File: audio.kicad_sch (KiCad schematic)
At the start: 33 parts, among them IC1 ES9218PQ, J5 SJ2-35954B-SMT-TR, Y2 ECS-2520SMV-500-GP-TR

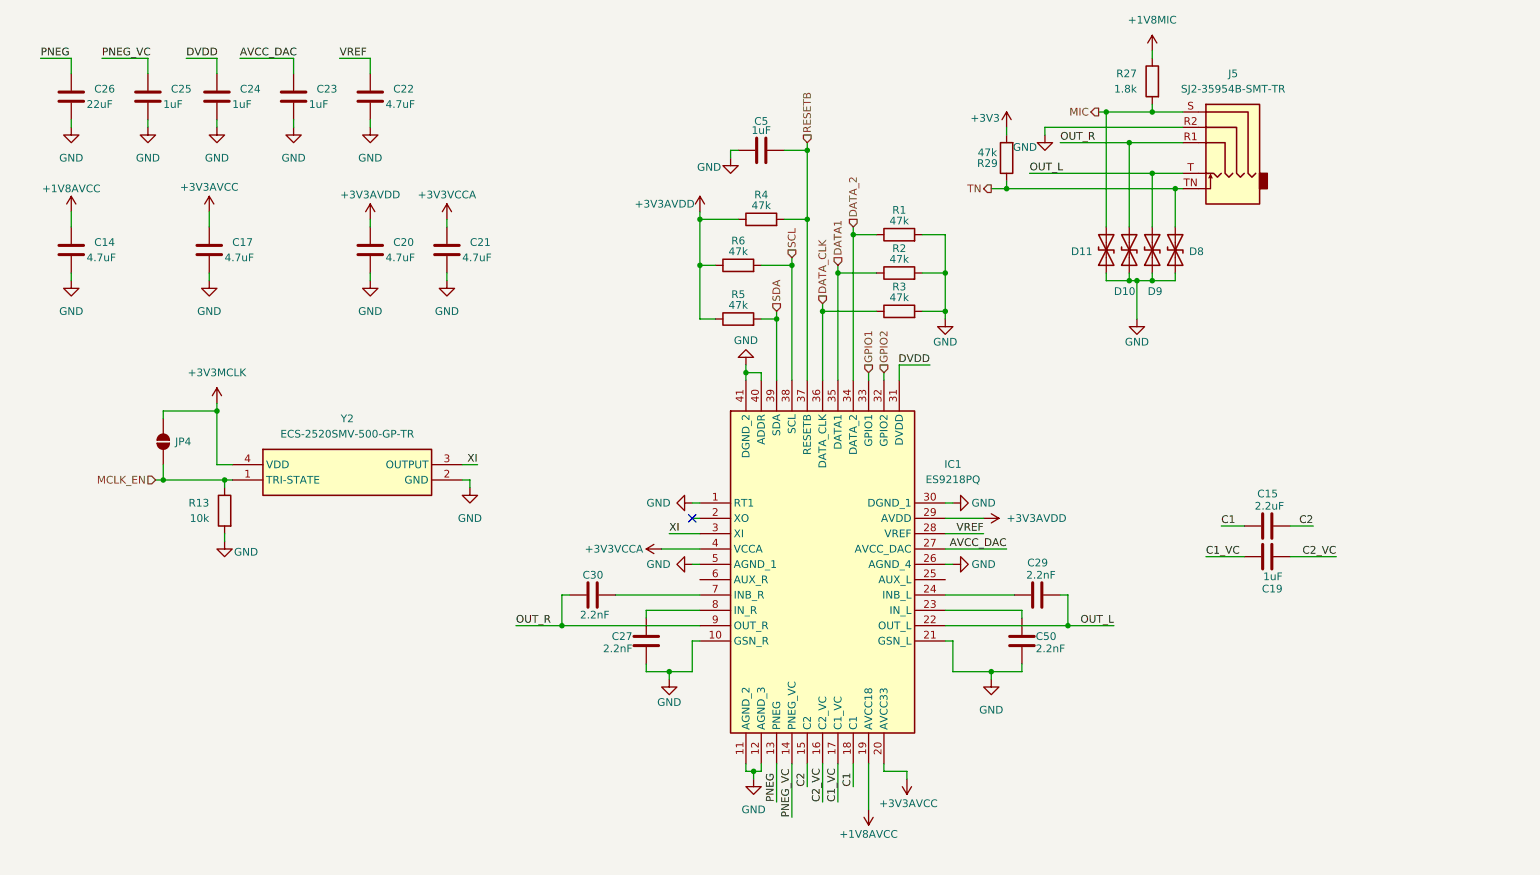
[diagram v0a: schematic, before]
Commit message: segmented schematci
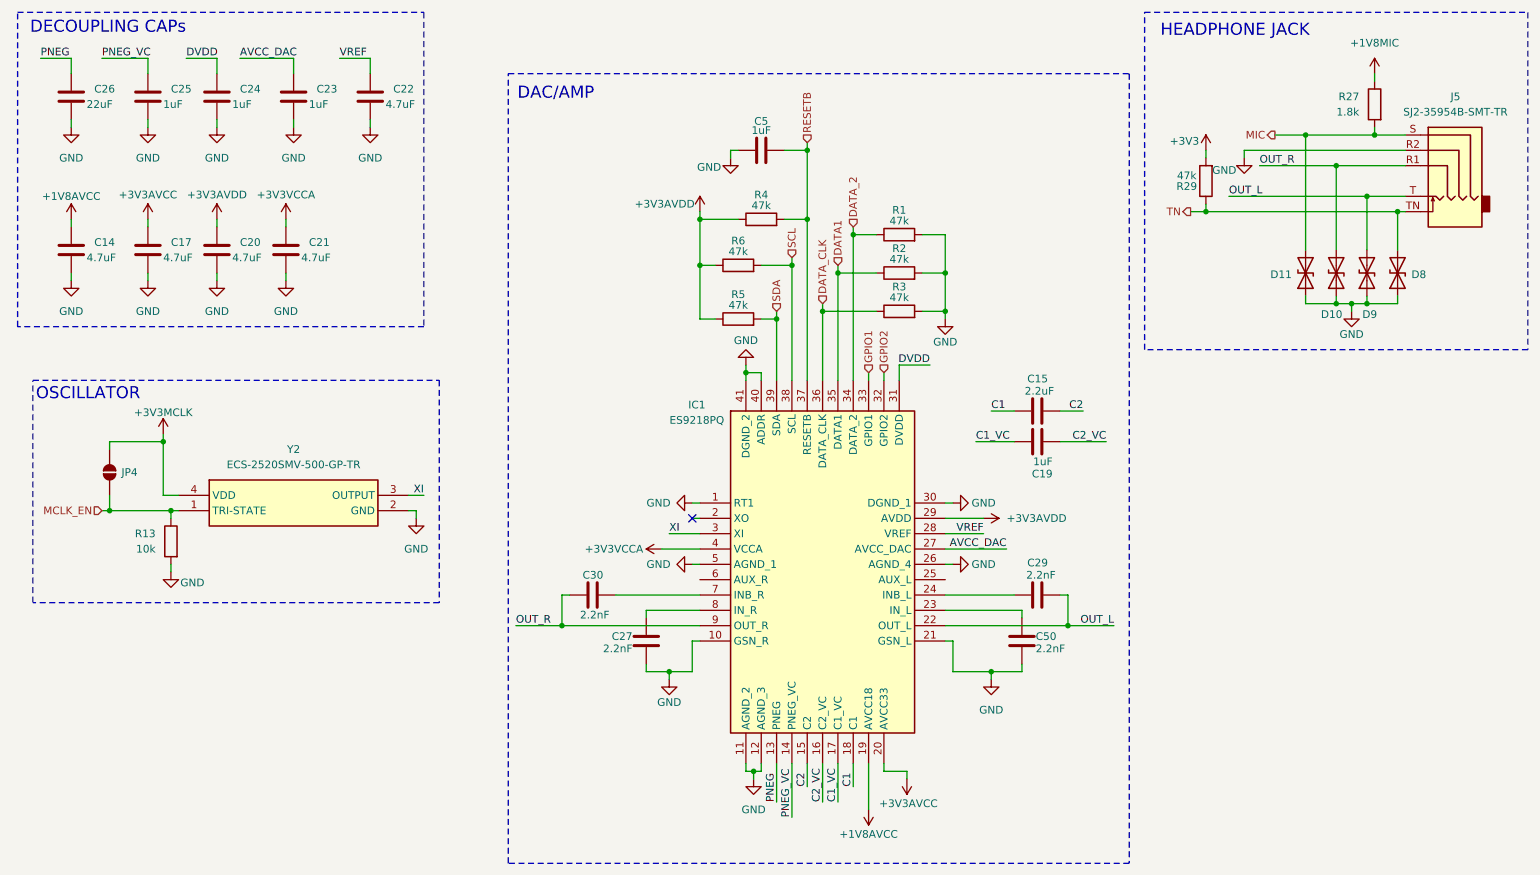
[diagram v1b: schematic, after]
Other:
- note added: "DAC/AMP"
- note added: "DECOUPLING CAPs"
- note added: "HEADPHONE JACK"
- note added: "OSCILLATOR"
- moved on the sheet: C15, C17, C19, C20, C21, D10, D11, D8, D9, J5, JP4, R13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
